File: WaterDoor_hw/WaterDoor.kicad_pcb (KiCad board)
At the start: 2 copper layers, 78.7 x 70 mm, 96 parts, among them Q1 2N7002, Q2 MMBT2222, Q3 IRLMS9303, SW1 BUTTON, SW2 BUTTON, SW3 BUTTON, SW4 BUTTON, SW5 SWITCH_H, U1 MOC3061M, U2 BTB600

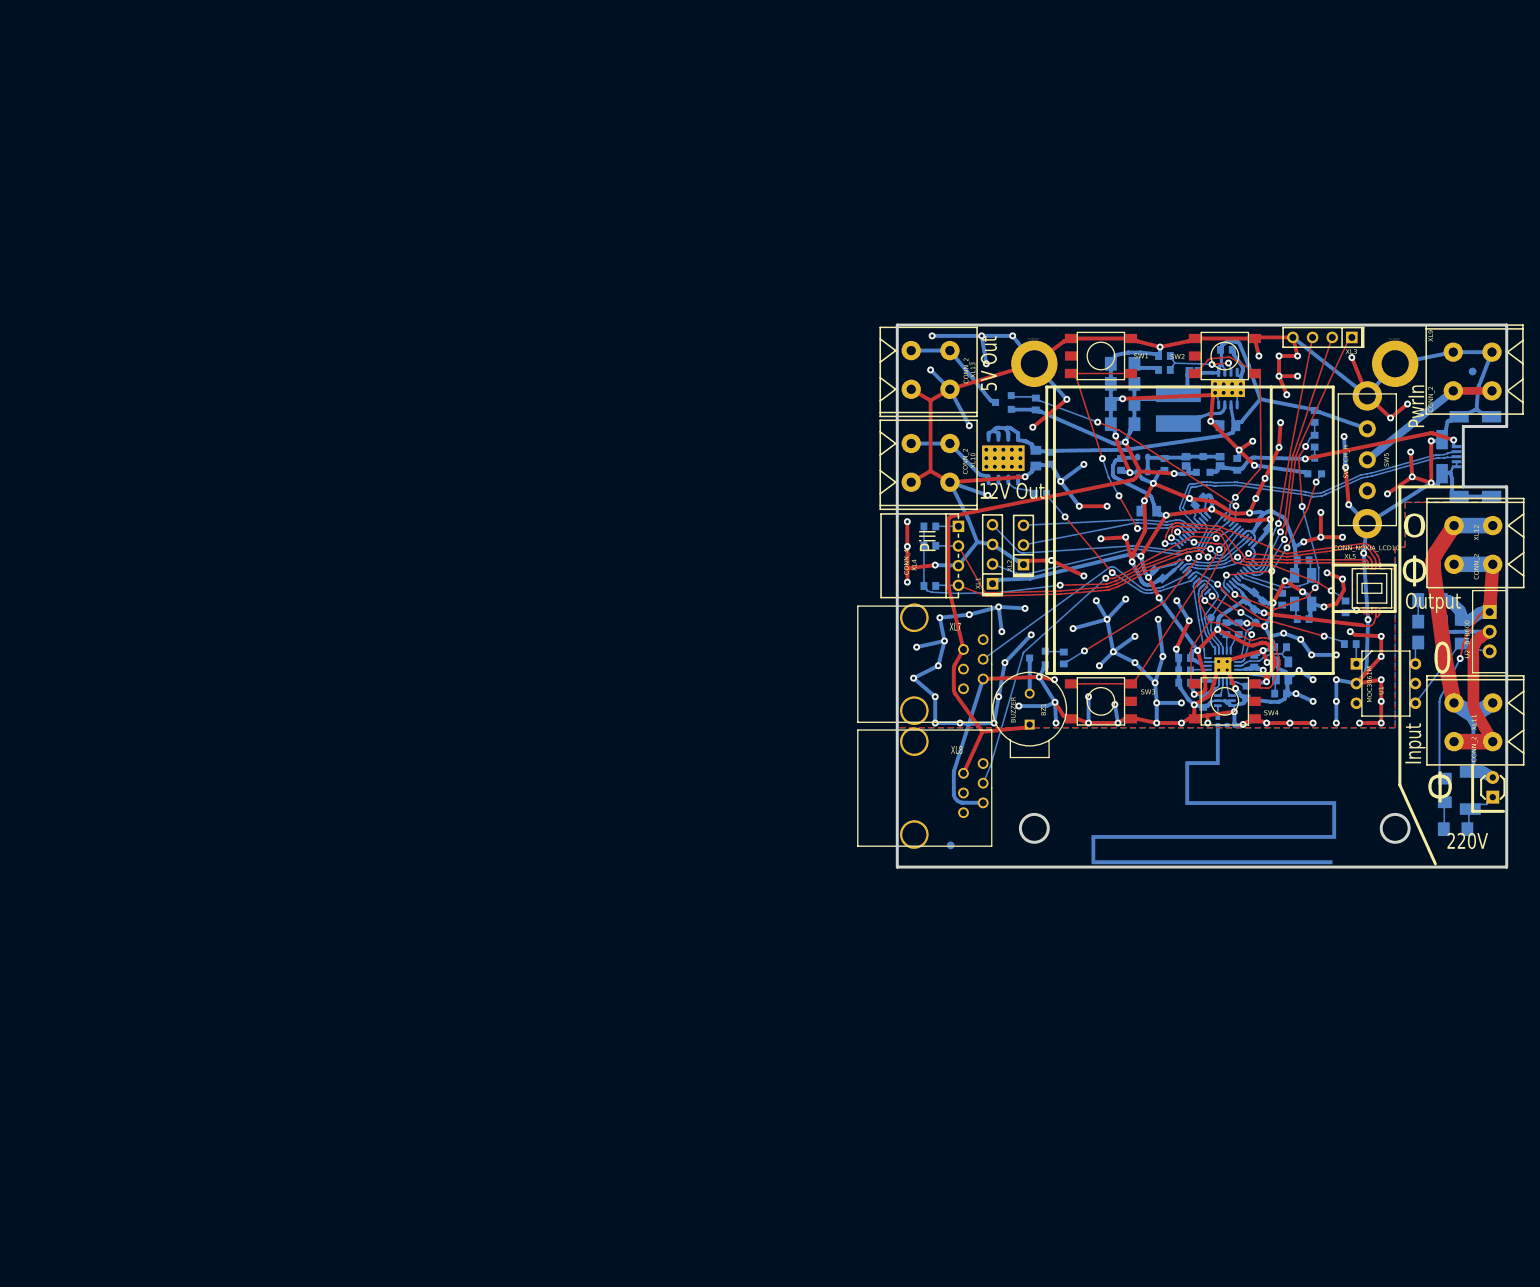
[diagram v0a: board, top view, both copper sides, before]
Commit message: + Main PCB ready for production
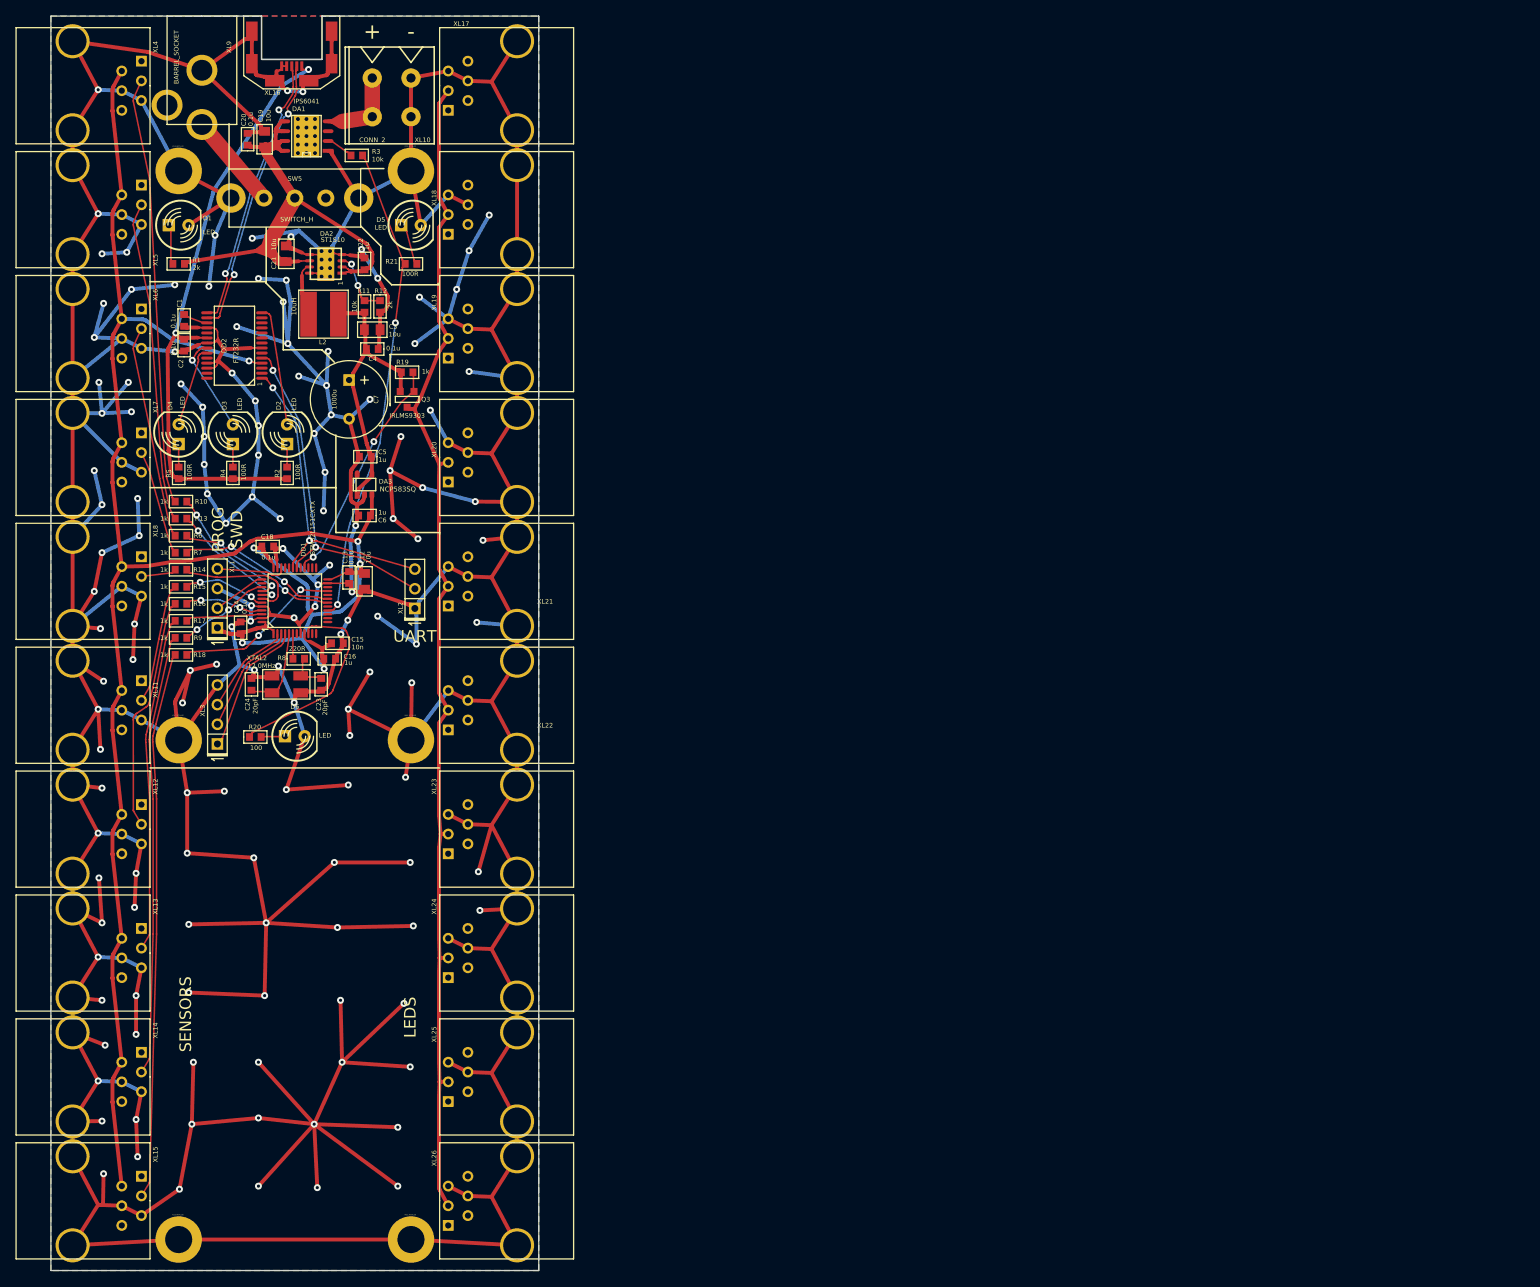
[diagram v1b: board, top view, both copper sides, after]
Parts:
- removed ANT1: ANT_PCB_MONO, ANT_868_MEANDER2
- removed BLN1: 0896BM15A0001, BALUN_JOHANSON868
- removed BZ1: BUZZER, BUZZER_HC0903
- removed C10, C9: 10pF, CAP_0603
- removed C11: 0.1u, CAP_0603
- removed C25, C26, C27, C28: 22u, CAP_1206
- removed C29, C31: 1u, CAP_0603
- removed C30: 0.01u, CAP_1206
- removed C8: 220pF, CAP_0603
- removed F1, F2, F3: FUSE0R, SMD0603_FUSE
- removed L1: 5.6nH, IND_0402
- removed Q1: 2N7002, SOT23
- removed Q2: MMBT2222, SOT23
- removed RP1, RP2: REFPOINT, REF_POINT_1MM
- removed SW1, SW2, SW3, SW4: BUTTON, BUTTON_6x6SMD
- removed TP1, TP2: TESTPOINT, TESTPOINT_1MM
- removed U1: MOC3061M, DIL6
- removed U2: BTB600, TO220
- removed XTAL1: 27MHz, CRYSTAL_03225C4
- added D4: LED, LEDs:Through-Hole-5mm, F.Cu at (69.5, 72.5)
- added D5: LED, LEDs:Through-Hole-5mm, F.Cu at (99.5, 45.5)
- added D6: LED, LEDs:Through-Hole-5mm, F.Cu at (84.5, 111.5)
- added HOLE3: HOLE_METALLED, PCB:Hole3_5_out6mm, F.Cu at (99.5, 38.5)
- added HOLE4: HOLE_METALLED, PCB:Hole3_5_out6mm, F.Cu at (69.5, 38.5)
- added HOLE5: HOLE_METALLED, PCB:Hole3_5_out6mm, F.Cu at (99.5, 112.0)
- added HOLE6: HOLE_METALLED, PCB:Hole3_5_out6mm, F.Cu at (69.5, 112.0)
- added R20: 100, Resistors:RES_0603, F.Cu at (79.4, 111.6)
- added R21: 100R, Resistors:RES_0603, F.Cu at (99.5, 50.5)
- added XL14: RJ11, Connectors:RJ11_TJ6_6P6C, F.Cu at (48.5, 155.5)
- added XL15: RJ11, Connectors:RJ11_TJ6_6P6C, F.Cu at (48.5, 171.5)
- added XL16: USB_MICRO_B, Connectors:USBmicro_MOLEX_WM17142, F.Cu at (84.1, 24.1)
- added XL17: RJ11, Connectors:RJ11_TJ6_6P6C, F.Cu at (120.5, 27.5)
- added XL18: RJ11, Connectors:RJ11_TJ6_6P6C, F.Cu at (120.5, 43.5)
- added XL19: RJ11, Connectors:RJ11_TJ6_6P6C, F.Cu at (120.5, 59.5)
- added XL20: RJ11, Connectors:RJ11_TJ6_6P6C, F.Cu at (120.5, 75.5)
- added XL21: RJ11, Connectors:RJ11_TJ6_6P6C, F.Cu at (120.5, 91.5)
- added XL22: RJ11, Connectors:RJ11_TJ6_6P6C, F.Cu at (120.5, 107.5)
- added XL23: RJ11, Connectors:RJ11_TJ6_6P6C, F.Cu at (120.5, 123.5)
- added XL24: RJ11, Connectors:RJ11_TJ6_6P6C, F.Cu at (120.5, 139.5)
- added XL25: RJ11, Connectors:RJ11_TJ6_6P6C, F.Cu at (120.5, 155.5)
- added XL26: RJ11, Connectors:RJ11_TJ6_6P6C, F.Cu at (120.5, 171.5)
- C1, C13, C14, C15, C16, C18, C20, C22, C23, C24: footprint CAP_0603 -> Capacitors:CAP_0603; moved to F.Cu
- C12, C19, C21: footprint CAP_0805 -> Capacitors:CAP_0805; moved to F.Cu
- C2: value 1.8pF -> 0.1u; footprint CAP_0402 -> Capacitors:CAP_0603; moved to F.Cu
- C3: value 220pF -> 10u; footprint CAP_0603 -> Capacitors:CAP_0805; moved to F.Cu
- C4: value 10n -> 0.1u; footprint CAP_0603 -> Capacitors:CAP_0603; moved to F.Cu
- C5: value 3.3pF -> 1u; footprint CAP_0603 -> Capacitors:CAP_0603; moved to F.Cu
- C6: value 10n -> 1u; footprint CAP_0603 -> Capacitors:CAP_0603; moved to F.Cu
- C7: value 0.1u -> 1000u; footprint CAP_0603 -> Capacitors:CAP_10xxR; moved to F.Cu
- D1: value BAXXXC -> LED; footprint SOT23 -> LEDs:Through-Hole-5mm; moved to F.Cu
- D2: value SM4007 -> LED; footprint DIODE_MELF_DO213AB -> LEDs:Through-Hole-5mm; moved to F.Cu
- D3: footprint LED-3MM -> LEDs:Through-Hole-5mm
- DA1: footprint SO8HEATSINK -> SO_DIL_TSSOP:SO8HEATSINK; moved to F.Cu
- DA2: footprint DFN8 -> QFN_DFN:DFN8; moved to F.Cu
- DA3: footprint SC82AB -> SOT:SOT23-5; moved to F.Cu
- DD1: footprint LQFP48 -> LQFP_TQFP:LQFP48; moved to F.Cu
- DD2: value CC1101 -> FT232R; footprint QFN20 -> SO_DIL_TSSOP:SSOP28; moved to F.Cu
- HOLE1, HOLE2: footprint Hole3_5_out6mm -> PCB:Hole3_5_out6mm
- L2: footprint IND_SR0604 -> Inductors:IND_SR0604; moved to F.Cu
- Q3: footprint SOT23 -> SOT:SOT23-3; moved to F.Cu
- R1: value 51R -> 2k; footprint RES_0603 -> Resistors:RES_0603; moved to F.Cu
- R10: value 10k -> 1k; footprint RES_0603 -> Resistors:RES_0603; moved to F.Cu
- R11, R12, R19, R3, R8: footprint RES_0603 -> Resistors:RES_0603; moved to F.Cu
- R13: value 150R -> 1k; footprint RES_0603 -> Resistors:RES_0603; moved to F.Cu
- R14: value 200k -> 1k; footprint RES_1206 -> Resistors:RES_0603; moved to F.Cu
- R15: value 200R -> 1k; footprint RES_1206 -> Resistors:RES_0603; moved to F.Cu
- R16: value 39R -> 1k; footprint RES_1206 -> Resistors:RES_0603; moved to F.Cu
- R17, R18: value 51k -> 1k; footprint RES_1206 -> Resistors:RES_0603; moved to F.Cu
- R2: value 56k -> 100R; footprint RES_0603 -> Resistors:RES_0603; moved to F.Cu
- R4: value 1k -> 100R; footprint RES_0603 -> Resistors:RES_0603; moved to F.Cu
- R5: value 4K7 -> 100R; footprint RES_0603 -> Resistors:RES_0603; moved to F.Cu
- R6: value 4K7 -> 1k; footprint RES_0603 -> Resistors:RES_0603; moved to F.Cu
- R7: value 150 -> 1k; footprint RES_0603 -> Resistors:RES_0603; moved to F.Cu
- R9: value 43k -> 1k; footprint RES_0603 -> Resistors:RES_0603; moved to F.Cu
- SW5: footprint SWITCH_SS9 -> BtnsSwitches:SW_SS9
- XL1, XL3: footprint CONN_PLS-4 -> Connectors:PLS-4
- XL10: footprint SPRING_TERM_XY124V_A_2 -> Connectors:SPRING_TERM_XY124V_A_2
- XL11, XL12, XL13: value CONN_2 -> RJ11; footprint SPRING_TERM_XY124V_A_2 -> Connectors:RJ11_TJ6_6P6C
- XL2: footprint CONN_PLS-3 -> Connectors:PLS-3
- XL4: value CONN_4 -> RJ11; footprint CONN_PBS_4R -> Connectors:RJ11_TJ6_6P6C
- XL5: value CONN_NOKIA_LCD10 -> RJ11; footprint CONN_NOKIA1101_LCD -> Connectors:RJ11_TJ6_6P6C
- XL6: value USB_MICRO_B -> RJ11; footprint USBmicro_MOLEX_WM17142 -> Connectors:RJ11_TJ6_6P6C; moved to F.Cu
- XL7, XL8: footprint RJ11_TJ6_6P6C -> Connectors:RJ11_TJ6_6P6C
- XL9: value CONN_2 -> BARREL_SOCKET; footprint SPRING_TERM_XY124V_A_2 -> Connectors:Barrel
- XTAL2: footprint CRYSTAL_0503x4-4 -> Quartz:0503x4-4; moved to F.Cu
- moved HOLE2 193.6 mm to (69.5, 176.5)
- moved XL12 191.7 mm to (48.5, 123.5), turned to 0 degrees
- moved XL11 188.2 mm to (48.5, 107.5), turned to 0 degrees
- moved XL6 187.6 mm to (48.5, 59.5), turned to 0 degrees
- moved XL5 181.8 mm to (48.5, 43.5), turned to 0 degrees
- moved D3 169.0 mm to (76.5, 72.5)
- moved XL9 167.2 mm to (72.5, 32.5), turned to 270 degrees
- moved R18 166.1 mm to (69.8, 101.0)
- moved R14 165.6 mm to (69.8, 90.0), turned to 0 degrees
- moved R17 164.7 mm to (69.8, 96.6), turned to 0 degrees
- moved R15 161.5 mm to (69.8, 92.2)
- moved R16 161.3 mm to (69.8, 94.4), turned to 0 degrees
- moved D2 159.6 mm to (83.5, 72.5)
- moved R1 157.1 mm to (69.5, 50.5), turned to 180 degrees
- moved XL3 152.1 mm to (74.5, 112.5), turned to 90 degrees
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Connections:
- C1 pad 1: VCC -> Net-(C1-Pad1)
- C19 pad 1: +BATT -> +12V
- C2 pad 1: N-0000073 -> GND
- C2 pad 2: GND -> /+5V_FT
- C20 pad 1: +BATT -> +12V
- C21 pad 1: +BATT -> +12V
- C22 pad 1: +BATT -> +12V
- C3 pad 1: +3.3V -> GND
- C3 pad 2: GND -> +5V
- C4 pad 1: +3.3V -> GND
- C4 pad 2: GND -> +5V
- C5 pad 1: +3.3V -> +5V
- C7 pad 1: +3.3V -> +5V
- D2 pad A: GNDPWR -> Net-(D2-PadA)
- D2 pad C: N-0000017 -> Net-(D2-PadC)
- D3 pad A: N-0000017 -> Net-(D3-PadA)
- D3 pad C: GNDPWR -> Net-(D3-PadC)
- DA1 pad 5: +BATT -> +12V
- DA1 pad 6: +BATT -> +12V
- DA1 pad 7: +BATT -> +12V
- DA1 pad 8: +BATT -> +12V
- DA2 pad 1: +BATT -> +12V
- DA2 pad 2: +BATT -> +12V
- DA2 pad 6: +BATT -> +12V
- DA3 pad 1: N-0000051 -> +5V
- DA3 pad 4: N-0000051 -> +5V
- DD1 pad 10: N-0000059 -> Net-(DD1-Pad10)
- DD1 pad 11: N-0000057 -> (no net)
- DD1 pad 12: /CC_GDO2 -> (no net)
- DD1 pad 13: /CC_GDO0 -> (no net)
- DD1 pad 14: /CC_CS -> (no net)
- DD1 pad 15: /CC_SCK -> (no net)
- DD1 pad 16: /CC_MISO -> /12V_CTRL
- DD1 pad 17: /CC_MOSI -> (no net)
- DD1 pad 18: /12V_CTRL -> /SNS3R
- DD1 pad 19: /220V_CTRL -> /SNS4R
- DD1 pad 20: /SNS1 -> (no net)
- DD1 pad 21: /LCD_SDA -> /SNS10R
- DD1 pad 22: /LCD_XRES -> (no net)
- DD1 pad 25: /LCD_SCLK -> (no net)
- DD1 pad 26: /LCD_XCS -> (no net)
- DD1 pad 27: /LCD_BCKLT -> (no net)
- DD1 pad 28: /BTN4 -> /LEDS_CTRL
- DD1 pad 29: /BTN1 -> (no net)
- DD1 pad 32: /USB_DM -> (no net)
- DD1 pad 33: /USB_DP -> (no net)
- DD1 pad 38: /BTN2 -> (no net)
- DD1 pad 39: /Buzzer -> /SNS9R
- DD1 pad 40: /5V_CTRL -> /SNS1R
- DD1 pad 41: /SNS2 -> /SNS2R
- DD1 pad 42: /BTN3 -> /SNS5R
- DD1 pad 43: /PeriphPwr -> /SNS6R
- DD1 pad 45: /P_SCL -> /SNS7R
- DD1 pad 46: /P_SDA -> /SNS8R
- DD2 pad 1: /CC_SCK -> /UART_RX
- DD2 pad 10: N-0000077 -> (no net)
- DD2 pad 11: +3.3V -> (no net)
- DD2 pad 12: /RF1 -> (no net)
- DD2 pad 13: /RF2 -> (no net)
- DD2 pad 14: +3.3V -> Net-(D2-PadC)
- DD2 pad 15: +3.3V -> Net-(DD2-Pad15)
- DD2 pad 16: GND -> Net-(DD2-Pad16)
- DD2 pad 17: N-0000072 -> Net-(C1-Pad1)
- DD2 pad 18: +3.3V -> GND
- DD2 pad 19: GND -> (no net)
- DD2 pad 2: /CC_MISO -> (no net)
- DD2 pad 20: /CC_MOSI -> /+5V_FT
- DD2 pad 3: /CC_GDO2 -> (no net)
- DD2 pad 5: N-0000082 -> /UART_TX
- DD2 pad 6: /CC_GDO0 -> (no net)
- DD2 pad 7: /CC_CS -> GND
- DD2 pad 8: N-0000076 -> (no net)
- DD2 pad 9: +3.3V -> (no net)
- Q3 pad 1: /5V_CTRL -> /LEDS_CTRL
- Q3 pad 3: N-000006 -> /LEDS_OUT
- R1 pad 1: N-0000014 -> +12V
- R1 pad 2: /LCD_BCKLT -> Net-(D1-PadA)
- R10 pad 1: N-0000059 -> /SNS1
- R10 pad 2: N-0000058 -> /SNS1R
- R13 pad 1: /220V_CTRL -> /SNS2
- R13 pad 2: N-0000016 -> /SNS2R
- R14 pad 1: N-000004 -> /SNS5
- R14 pad 2: /OUT_220V -> /SNS5R
- R15 pad 1: N-000003 -> /SNS6
- R15 pad 2: /In_220 -> /SNS6R
- R16 pad 1: /In_220 -> /SNS7
- R16 pad 2: N-000005 -> /SNS7R
- R17 pad 1: /OUT_220V -> /SNS8
- R17 pad 2: N-0000018 -> /SNS8R
- R18 pad 1: N-0000018 -> /SNS10
- R18 pad 2: N-0000017 -> /SNS10R
- R19 pad 2: /5V_CTRL -> /LEDS_CTRL
- R2 pad 1: N-0000072 -> /+5V_FT
- R2 pad 2: GND -> Net-(D2-PadA)
- R4 pad 1: /Buzzer -> /+5V_FT
- R4 pad 2: N-0000022 -> Net-(D3-PadA)
- R5 pad 1: /P_SCL -> /+5V_FT
- R5 pad 2: /PeriphPwr -> Net-(D4-PadA)
- R6 pad 1: /P_SDA -> /SNS3
- R6 pad 2: /PeriphPwr -> /SNS3R
- R7 pad 1: /PeriphPwr1 -> /SNS4
- R7 pad 2: /PeriphPwr -> /SNS4R
- R9 pad 1: N-0000059 -> /SNS9
- R9 pad 2: +BATT -> /SNS9R
- SW5 pad 1: +BATT -> /PWR_IN
- SW5 pad 2: N-0000036 -> +12V
- XL10 pad 1: /OUT_12V -> GND
- XL10 pad 2: GND -> /OUT_12V
- XL11 pad 1: /In_220 -> (no net)
- XL11 pad 2: GNDPWR -> +3.3V
- XL12 pad 1: /OUT_220V -> (no net)
- XL12 pad 2: GNDPWR -> +3.3V
- XL13 pad 1: N-000006 -> (no net)
- XL13 pad 2: GND -> +3.3V
- XL4 pad 1: /PeriphPwr1 -> (no net)
- XL4 pad 2: /P_SCL -> +3.3V
- XL4 pad 3: GND -> /SNS1
- XL4 pad 4: /P_SDA -> GND
- XL5 pad 1: /LCD_SCLK -> (no net)
- XL5 pad 2: /LCD_SDA -> +3.3V
- XL5 pad 3: GND -> /SNS2
- XL5 pad 4: /LCD_XCS -> GND
- XL5 pad 5: /LCD_XRES -> GND
- XL5 pad 6: N-0000014 -> (no net)
- XL6 pad 1: VCC -> (no net)
- XL6 pad 2: /USB_DM -> +3.3V
- XL6 pad 3: /USB_DP -> /SNS3
- XL7 pad 2: +5V -> +3.3V
- XL7 pad 3: /SNS1 -> /SNS4
- XL7 pad 4: (no net) -> GND
- XL7 pad H: (no net) -> GND
- XL8 pad 2: +5V -> +3.3V
- XL8 pad 3: /SNS2 -> /SNS5
- XL8 pad 4: (no net) -> GND
- XL8 pad H: (no net) -> GND
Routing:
- net GND: track 835.3 -> 1575.1 mm, vias 141 -> 144
- net /LEDS_OUT: track 0.00 -> 154.2 mm
- net +3.3V: track 168.0 -> 277.8 mm, vias 12 -> 6
- net +5V: track 119.1 -> 37.2 mm, vias 2 -> 0
- net /+5V_FT: track 0.00 -> 79.3 mm, vias 0 -> 2
- net +BATT: track 77.4 -> 0.00 mm
- net +12V: track 0.00 -> 73.0 mm
- net /SNS10: track 0.00 -> 70.6 mm
- net /SNS9: track 0.00 -> 57.0 mm
- net /PeriphPwr: track 51.8 -> 0.00 mm, vias 2 -> 0
- net GNDPWR: track 48.2 -> 0.00 mm
- net /P_SCL: track 45.9 -> 0.00 mm, vias 1 -> 0
- net /OUT_220V: track 43.4 -> 0.00 mm, vias 1 -> 0
- net /SNS8: track 0.00 -> 43.2 mm
- net /BTN4: track 42.7 -> 0.00 mm, vias 1 -> 0
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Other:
- board size 78.7 x 70 mm -> 63 x 162 mm
- net class WideWide removed
- rule via_min_size: 0.889 -> 0.4
- board text added: "+"
- board text added: "-"
- board text added: "LEDS"
- board text added: "PROG SWD"
- board text added: "SENSORS"
- board text added: "UART"
- board text removed: "0"
- board text removed: "12V Out"
- board text removed: "12V Pwr"
- board text removed: "220V"
- board text removed: "220V Output indication"
- board text removed: "220V control"
- board text removed: "220V domain"
- board text removed: "3V3 Pwr"
- board text removed: "5V"
- board text removed: "5V Out"
- board text removed: "Battery measurement"
- board text removed: "Buzzer"
- board text removed: "Input"
- board text removed: "LCD Backlight"
- board text removed: "Optional pins"
- board text removed: "Output"
- board text removed: "Pill"
- board text removed: "Prog & debug"
- board text removed: "PwrIn"
- board text removed: "Quartz related"
- board text removed: "Radio"
- board text removed: "Solder the fuse if 12V pwr is not required"
- board text removed: "USB"
- board text removed: "Ф"
